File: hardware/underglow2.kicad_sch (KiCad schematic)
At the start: 1 part, among them J101 J_Delphi_Sicma_24

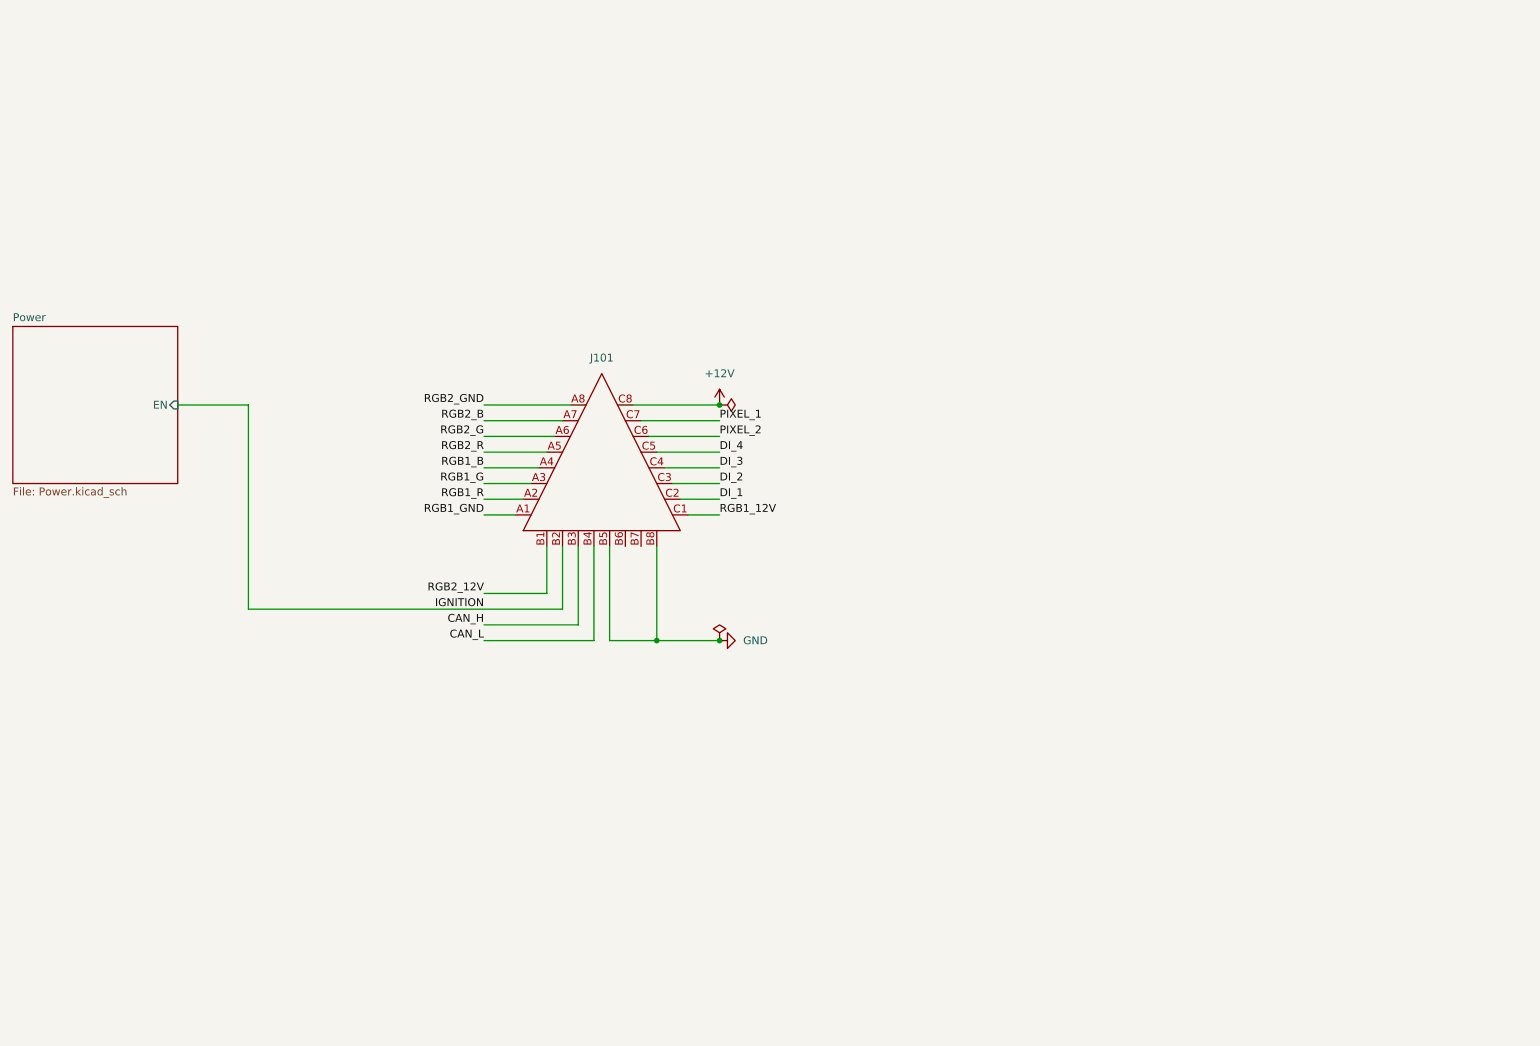
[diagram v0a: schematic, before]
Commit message: Schematic progress
Signed-off-by: Connor Rigby <connorr@hey.com>
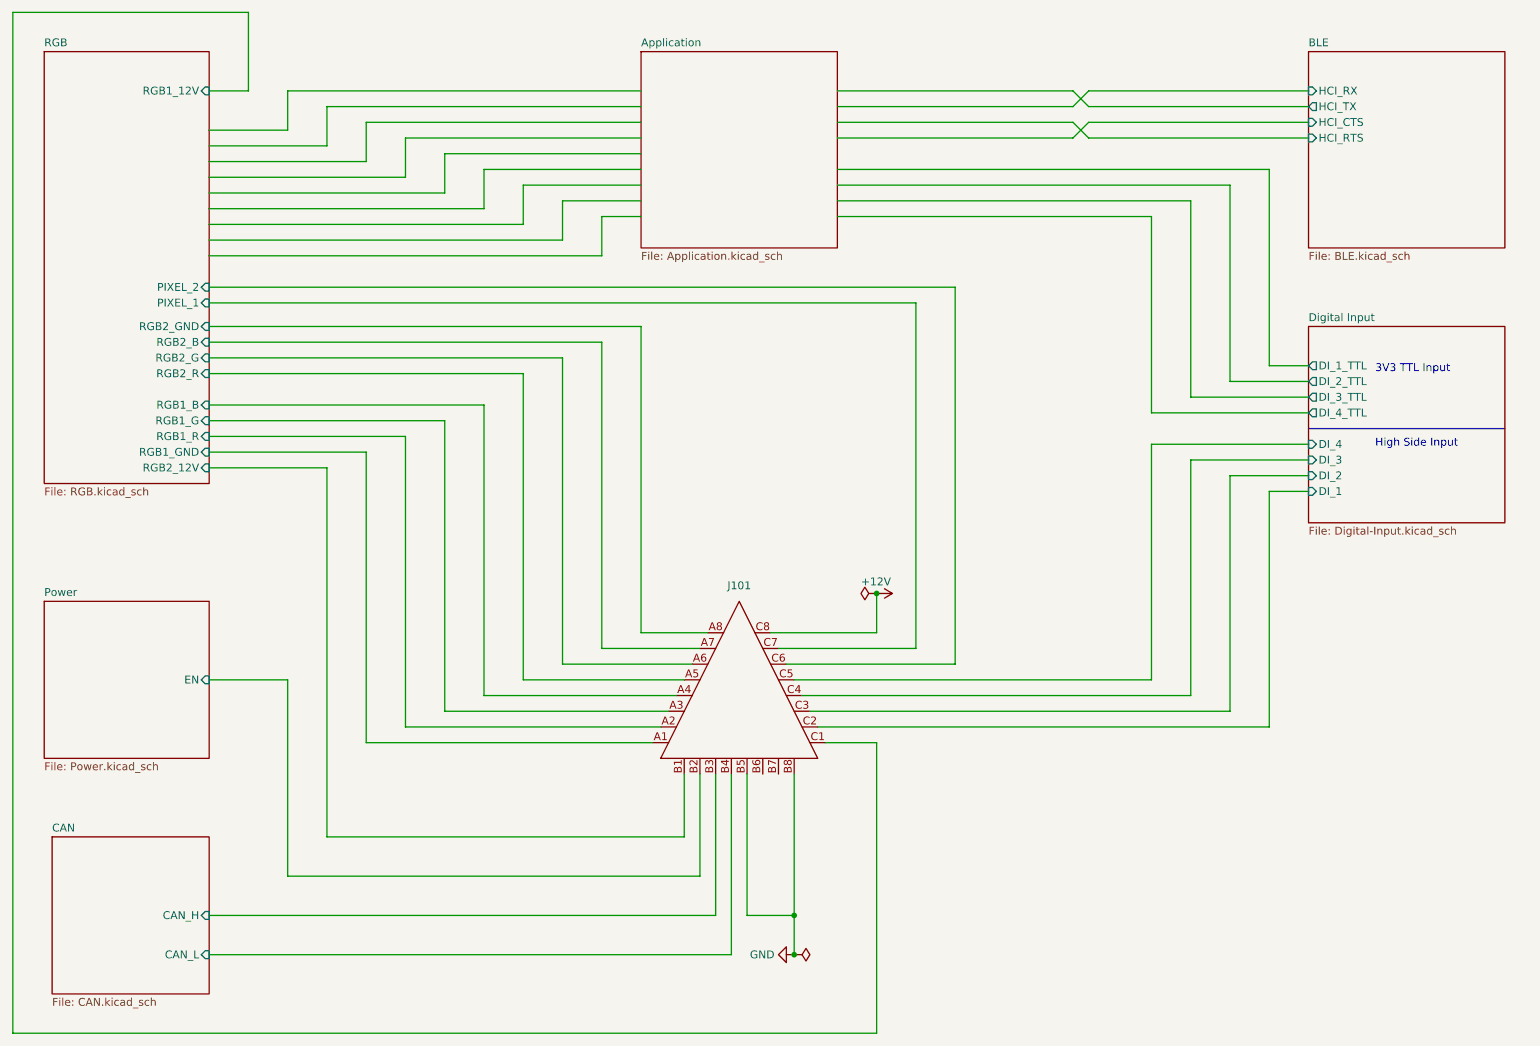
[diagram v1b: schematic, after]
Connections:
- net CAN_H renamed CAN/CAN_H
- net CAN_L renamed CAN/CAN_L
- net DI_1 renamed Digital Input/DI_1
- net DI_2 renamed Digital Input/DI_2
- net DI_3 renamed Digital Input/DI_3
- net DI_4 renamed Digital Input/DI_4
- net IGNITION renamed Power/EN
- net PIXEL_1 renamed RGB/PIXEL_1
- net PIXEL_2 renamed RGB/PIXEL_2
- net RGB1_12V renamed RGB/RGB1_12V
- net RGB1_B renamed RGB/RGB1_B
- net RGB1_G renamed RGB/RGB1_G
- net RGB1_GND renamed RGB/RGB1_GND
- net RGB1_R renamed RGB/RGB1_R
- net RGB2_12V renamed RGB/RGB2_12V
- net RGB2_B renamed RGB/RGB2_B
- net RGB2_G renamed RGB/RGB2_G
- net RGB2_GND renamed RGB/RGB2_GND
- net RGB2_R renamed RGB/RGB2_R
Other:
- added sheet Application (Application.kicad_sch)
- added sheet BLE (BLE.kicad_sch)
- added sheet CAN (CAN.kicad_sch)
- added sheet Digital Input (Digital-Input.kicad_sch)
- added sheet RGB (RGB.kicad_sch)
- note added: "3V3 TTL Input"
- note added: "High Side Input"
- moved on the sheet: J101
